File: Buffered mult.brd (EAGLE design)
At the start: 97.2 x 16.9 mm, 28 parts, among them IC1 OPA4171, IC4 OPA2171, J1 EURO_POWER_HEADERFAT_PADS

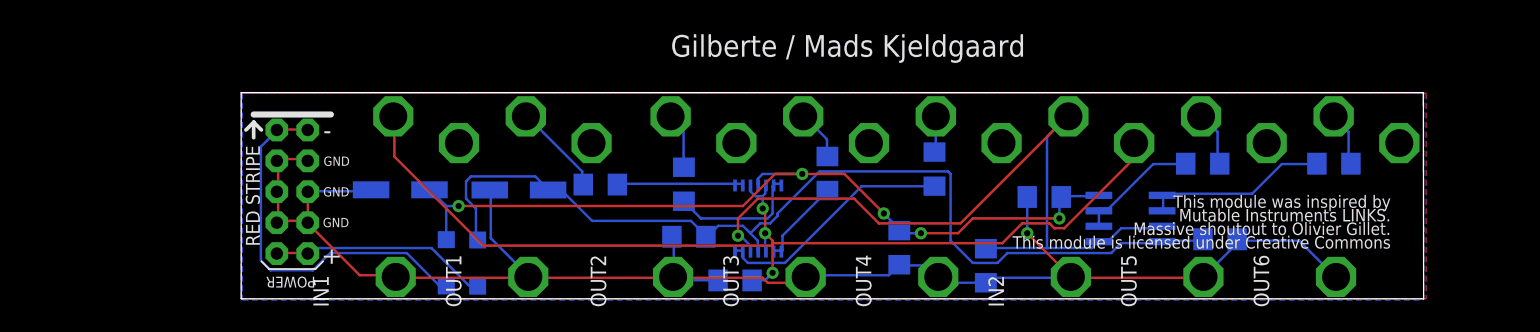
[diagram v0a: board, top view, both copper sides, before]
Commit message: small touchups
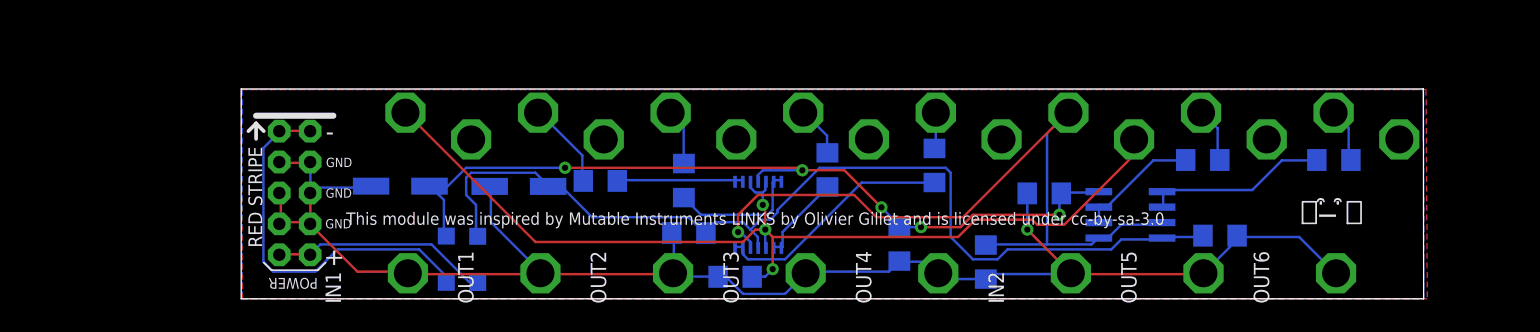
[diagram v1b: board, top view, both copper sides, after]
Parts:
- removed FRAME1: FRAME-LETTER, SparkFun-Aesthetics:CREATIVE_COMMONS
- moved IN1 1.04 mm to (13.7, -0.40)
- moved OUT1 1.04 mm to (24.6, -0.40)
- moved C13 0.30 mm to (22.8, 9.24)
- moved C2 0.30 mm to (66.0, 8.67)
- moved C3 0.30 mm to (80.5, 5.19)
- moved C7 0.30 mm to (36.8, 5.40)
- moved IC1 0.30 mm to (42.5, 6.90)
- moved IC4 0.30 mm to (73.1, 6.90)
- moved R1 0.30 mm to (36.4, 9.72)
- moved R4 0.30 mm to (57.0, 11.0)
- moved R5 0.30 mm to (79.0, 11.4)
- moved R6 0.30 mm to (89.8, 11.4)
- moved D2 0.30 mm to (19.4, 3.24)
- moved R7 0.30 mm to (40.6, 1.81)
- moved IN2 0.30 mm to (68.2, -0.40)
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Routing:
- net N$5: track 84.4 -> 81.2 mm
- net GND: track 133.0 -> 130.4 mm
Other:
- board size 97.2 x 16.9 mm -> 97.2 x 17.2 mm
- board text added: "This module was inspired by Mutable Instruments LINKS by Olivier Gillet and is licensed under cc-by-sa-3.0"
- board text removed: "Gilberte / Mads Kjeldgaard"
- board text removed: "This module was inspired by Mutable Instruments LINKS. Massive shoutout to Olivier Gillet. This module is licensed under Creative Commons"
